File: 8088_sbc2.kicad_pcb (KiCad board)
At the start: 2 copper layers, 200 x 100 mm, 65 parts, among them P1 CONN_02X10, P2 JMP_USB_PWR, P3 USB_B, Q1 IRLML6402, SW1 SW_PUSH, U1 P8088, U11 74HC573, U12 74HC573, U13 74HC573, U14 74HC573, U15 74HC138, U16 74HC138, U17 74HC14_OWN, U18 74HC08, U19 74HC32, U2 28C64, U20 10xLEDBAR, U3 AS6C4008, U4 TL770xA, U5 16C550, U6 FT232RL, U7 OSC_SMALL

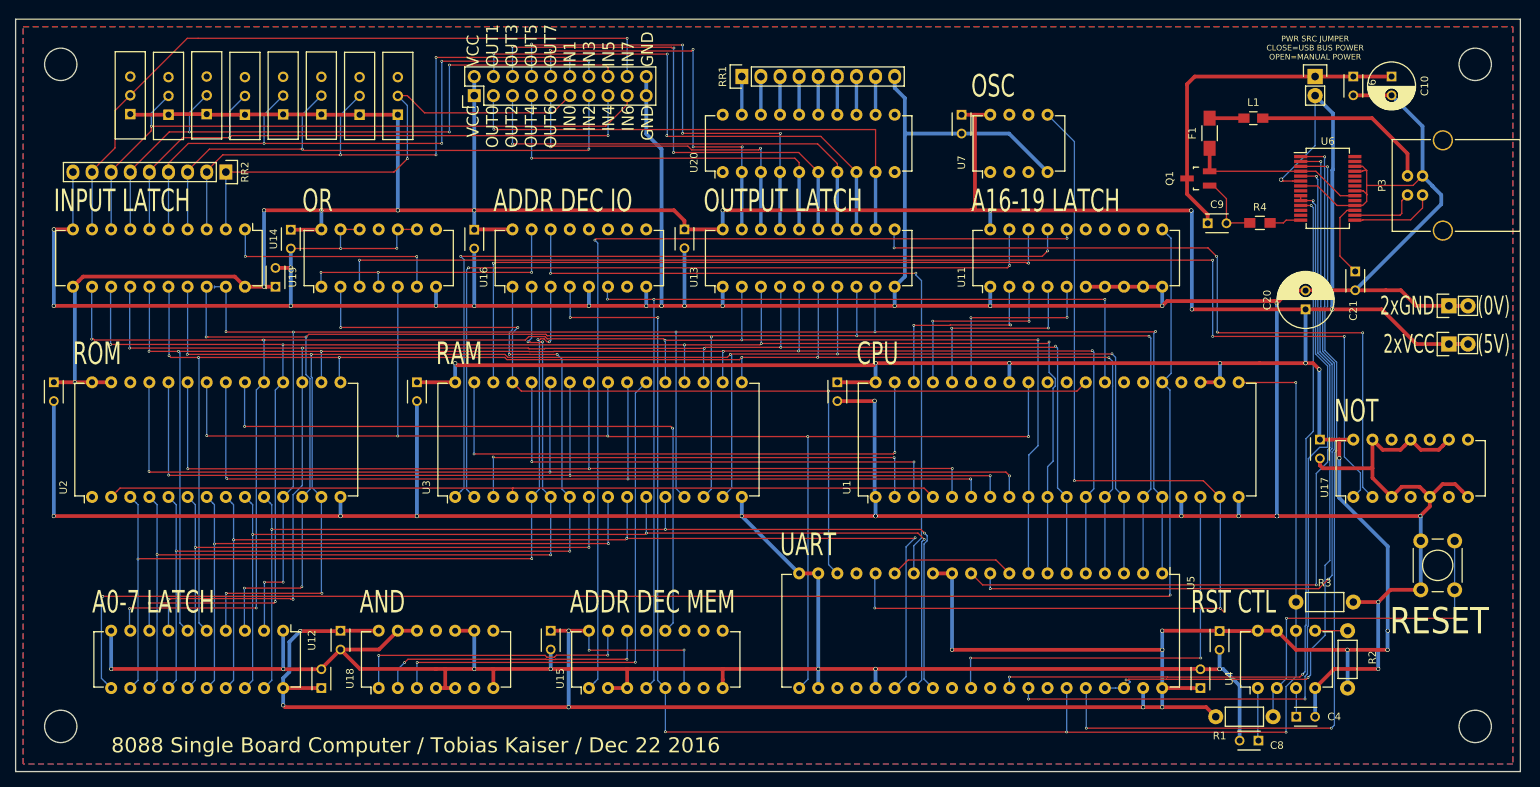
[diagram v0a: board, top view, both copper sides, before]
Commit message: test
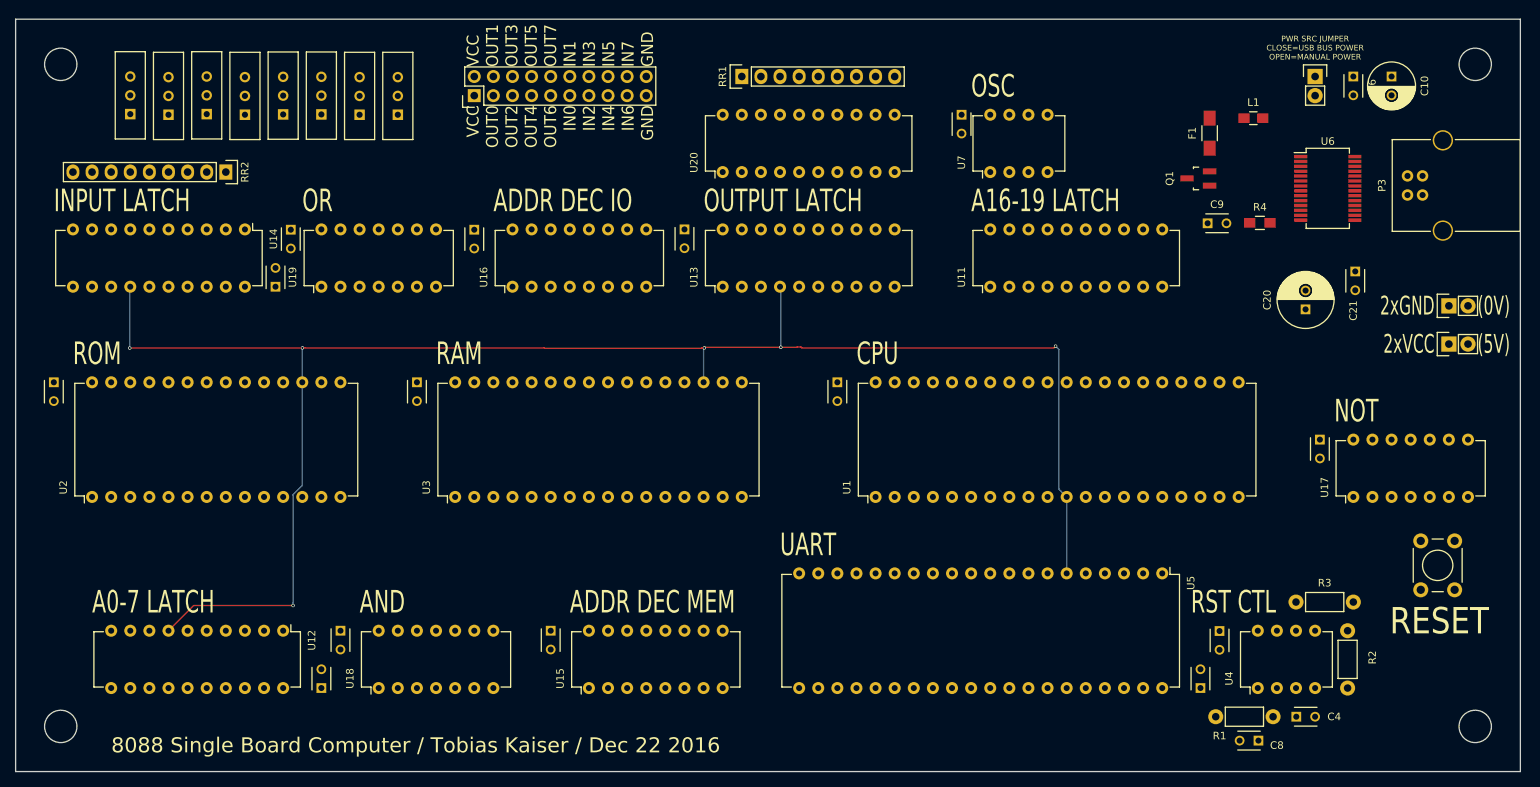
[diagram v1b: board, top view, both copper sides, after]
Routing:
- net GND: track 1033.4 -> 0.00 mm, vias 38 -> 0
- net VCC: track 853.9 -> 0.00 mm, vias 33 -> 0
- net /D2: track 241.0 -> 0.00 mm, vias 7 -> 0
- net /D1: track 240.1 -> 0.00 mm, vias 7 -> 0
- net /D0: track 235.4 -> 0.00 mm, vias 7 -> 0
- net /D7: track 233.4 -> 0.00 mm, vias 7 -> 0
- net /D6: track 231.8 -> 0.00 mm, vias 7 -> 0
- net /D4: track 218.7 -> 0.00 mm, vias 6 -> 0
- net /D3: track 216.8 -> 0.00 mm, vias 6 -> 0
- net /RES: track 214.3 -> 0.00 mm, vias 6 -> 0
- net /ALE: track 204.8 -> 0.00 mm, vias 2 -> 0
- net /nRD: track 184.5 -> 0.00 mm, vias 5 -> 0
- net /nIODEV0_WREN: track 167.2 -> 0.00 mm, vias 4 -> 0
- net /A2: track 143.6 -> 0.00 mm, vias 3 -> 0
- net /A8: track 141.3 -> 0.00 mm, vias 3 -> 0
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- removed copper zone on B.Cu, net GND
- removed copper zone on F.Cu, net GND

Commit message: shitty kicad fucked it up while saving. fuck it.
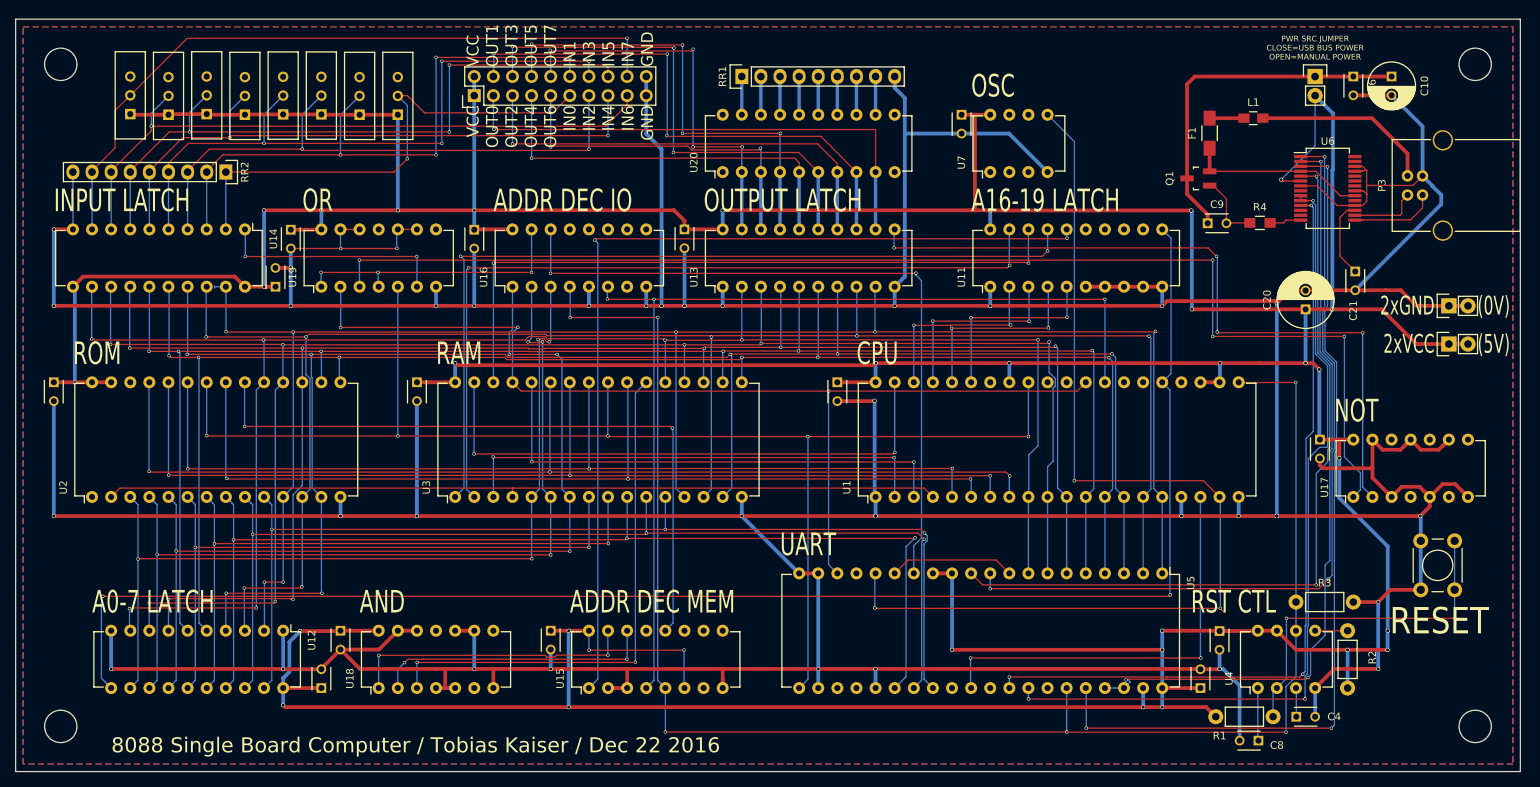
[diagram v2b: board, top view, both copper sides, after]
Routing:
- net GND: track 0.00 -> 1033.4 mm, vias 0 -> 38
- net VCC: track 0.00 -> 853.9 mm, vias 0 -> 33
- net /D2: track 0.00 -> 241.0 mm, vias 0 -> 7
- net /D1: track 0.00 -> 240.1 mm, vias 0 -> 7
- net /D0: track 0.00 -> 235.4 mm, vias 0 -> 7
- net /D7: track 0.00 -> 233.4 mm, vias 0 -> 7
- net /D6: track 0.00 -> 231.8 mm, vias 0 -> 7
- net /D4: track 0.00 -> 218.7 mm, vias 0 -> 6
- net /D3: track 0.00 -> 216.8 mm, vias 0 -> 6
- net /RES: track 0.00 -> 214.3 mm, vias 0 -> 6
- net /ALE: track 0.00 -> 204.8 mm, vias 0 -> 2
- net /nRD: track 0.00 -> 184.5 mm, vias 0 -> 5
- net /nIODEV0_WREN: track 0.00 -> 167.2 mm, vias 0 -> 4
- net /A2: track 0.00 -> 143.6 mm, vias 0 -> 3
- net /A8: track 0.00 -> 141.3 mm, vias 0 -> 3
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- added copper zone on B.Cu, net GND
- added copper zone on F.Cu, net GND
